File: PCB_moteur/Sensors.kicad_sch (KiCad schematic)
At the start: 13 parts, among them J4 Conn_01x04_Socket, J5 Conn_01x04_Socket, U11 MAX6612MXK, U5 INA125UA/2K5, U6 INA125UA/2K5

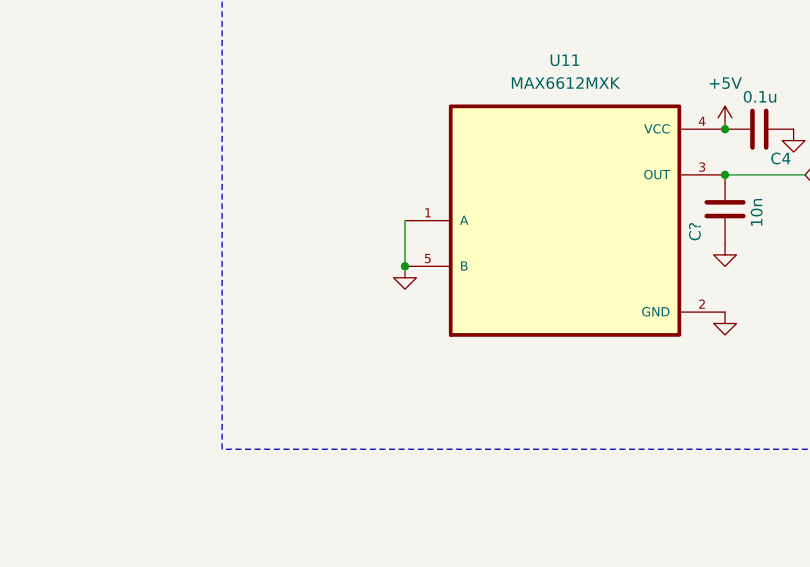
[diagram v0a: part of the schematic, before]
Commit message: fix: pyros resistors + typos +
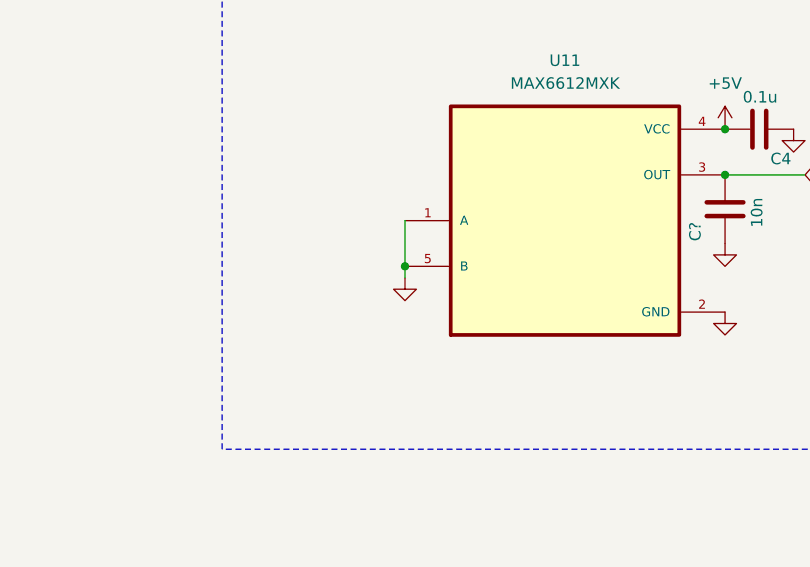
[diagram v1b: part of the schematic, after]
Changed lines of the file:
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@@
+	(wire
+		(pts
+			(xy 222.25 50.8) (xy 222.25 49.53)
+		)
+		(stroke
+			(width 0)
+			(type default)
+		)
+	)
 	(wire
 		(pts
@@
 	(symbol
 		(lib_id "power:GND")
-		(at 222.25 49.53 0)
+		(at 222.25 50.8 0)
 		(unit 1)
 		(exclude_from_sim no)
@@
 		(fields_autoplaced yes)
 		(property "Reference" "#PWR079"
+			(at 222.25 57.15 0)
+			(effects
+				(font
+					(size 1 1)
+				)
+				(hide yes)
+			)
+		)
+		(property "Value" "GND"
 			(at 222.25 55.88 0)
 			(effects
@@
 			)
 		)
-		(property "Value" "GND"
-			(at 222.25 54.61 0)
-			(effects
-				(font
-					(size 1 1)
-				)
-				(hide yes)
-			)
-		)
 		(property "Footprint" ""
-			(at 222.25 49.53 0)
+			(at 222.25 50.8 0)
 			(effects
 				(font
@@
 		)
 		(property "Datasheet" ""
-			(at 222.25 49.53 0)
+			(at 222.25 50.8 0)
 			(effects
 				(font
@@
 		)
 		(property "Description" ""
-			(at 222.25 49.53 0)
-			(effects
-				(font
+			(at 222.25 50.8 0)
+			(effects
+				(font
